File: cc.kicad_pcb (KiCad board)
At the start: 4 copper layers, 45.7 x 23.7 mm, 46 parts, among them J1 USB_OTG, J2 CONN_PWR, J3 CONN_DEBUG, J4 CONN_USART, P1 SMA, SW1 SW_Push, SW2 SW_Push, U1 TPS79333, U2 CC1200, U3 BALF-112X-02D3, U4 STM32L475RC, Y1 40MHz, Y2 8MHz(16pF)

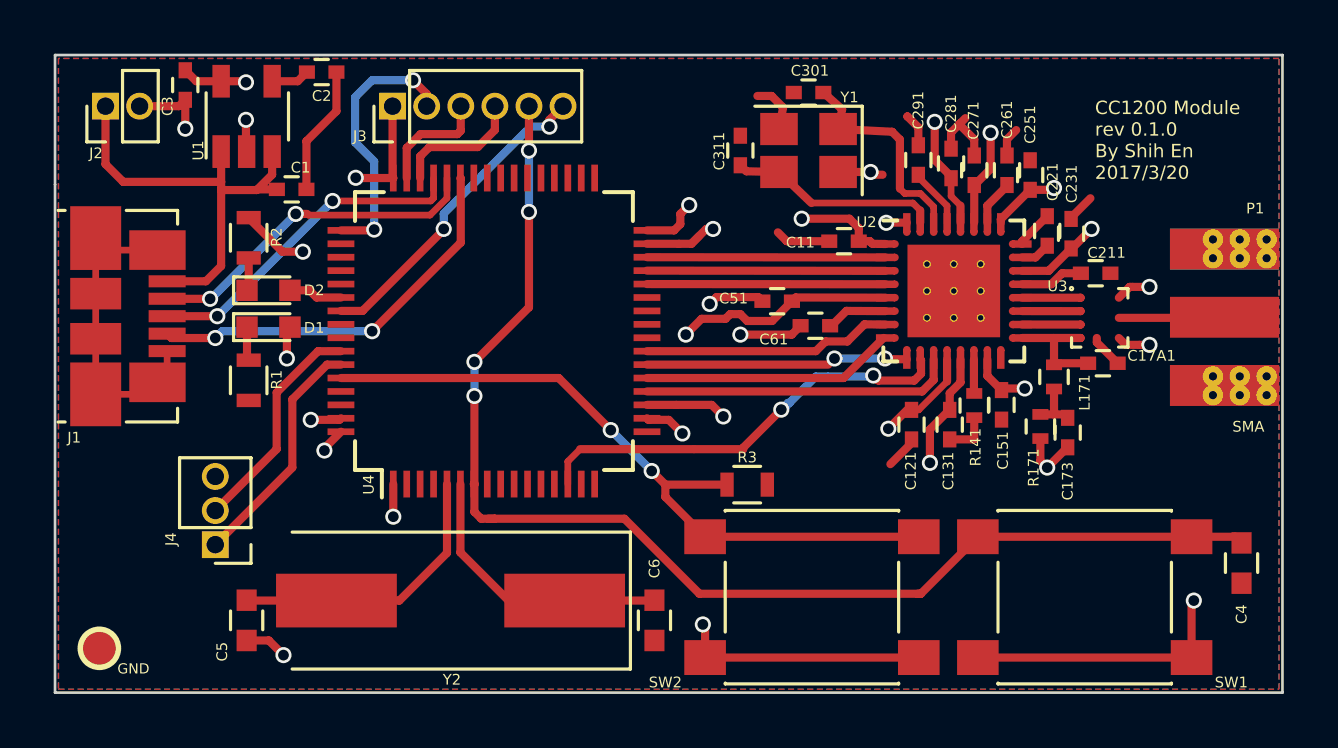
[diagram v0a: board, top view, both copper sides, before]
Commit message: Pre v0.1.0
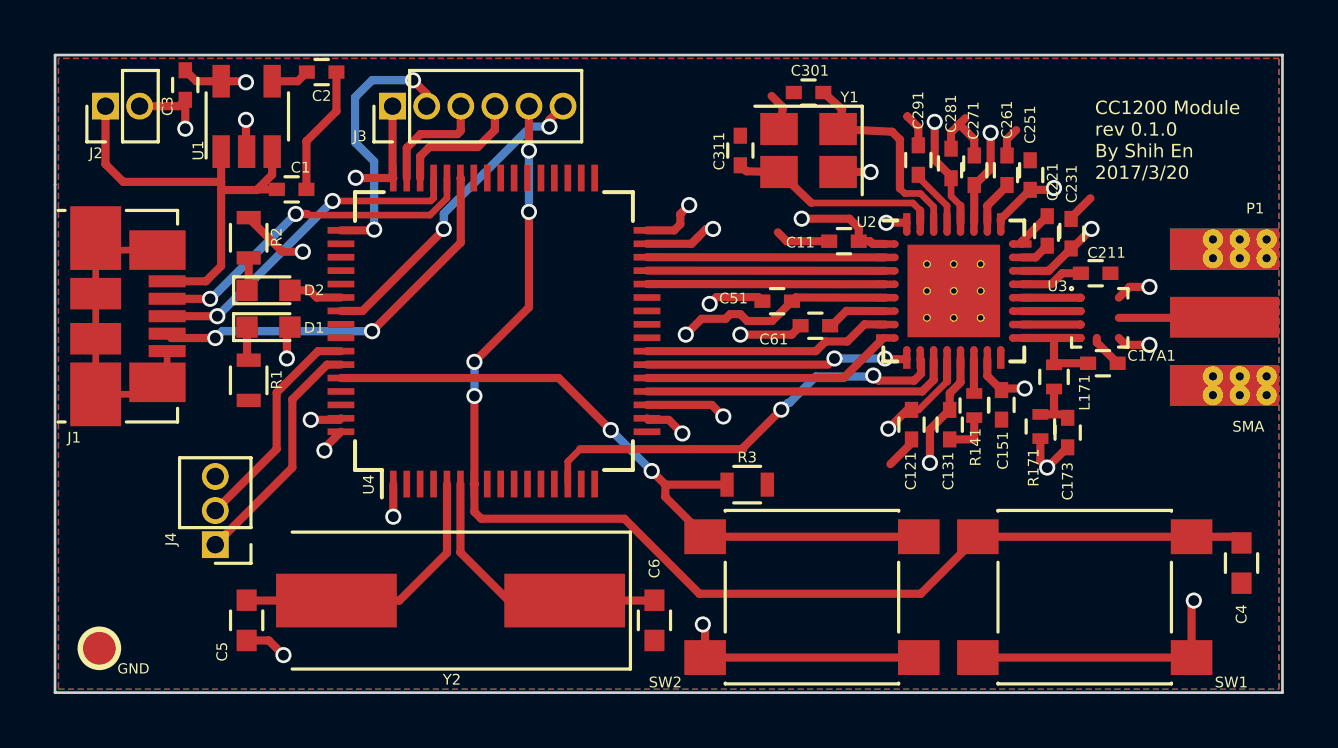
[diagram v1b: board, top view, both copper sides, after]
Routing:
- net GND: track 88.2 -> 87.3 mm
